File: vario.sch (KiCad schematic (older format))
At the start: 177 parts, among them J10 Conn_01x06, J11 Conn_01x04, J12 Conn_01x04, J13 Conn_01x04, J14 Conn_01x03, J15 Conn_01x04, J16 Conn_01x06, J17 Conn_01x06, J18 Conn_01x04, J19 Conn_01x04, J2 Conn_01x02, J20 Conn_01x06, J21 Conn_Coaxial, J22 USB_B_Micro, J23 USB_B_Micro, J24 Micro_SD_Card_Det_Hirose_DM3AT, J3 6339167-3, J6 Conn_01x06, J7 Conn_01x04, J8 Conn_01x04, J9 Conn_01x02, Q1 AO3401A, SW1 SW_MEC_5E, U1 STM32F407VGTx, U10 AMS1117-3.3, U11 HSCMRRN001PD2A3, U12 MS5611-01BA, U13 MAX3232ECPWR, U14 BLE_HM-11, U15 USBLC6-2SC6, U16 USBLC6-2SC6, U17 AMS1117-3.3, U18 HAMMOND_1593W, U2 MP2359DJ-LF-Z, U3 MP2359DJ-LF-Z, U4 L3GD20, U5 MTi-1IMU, U6 FXOS8700, U7 MS5611-01BA, U8 NEO-M9N, U9 TCAN332DR, Y1 16MHz

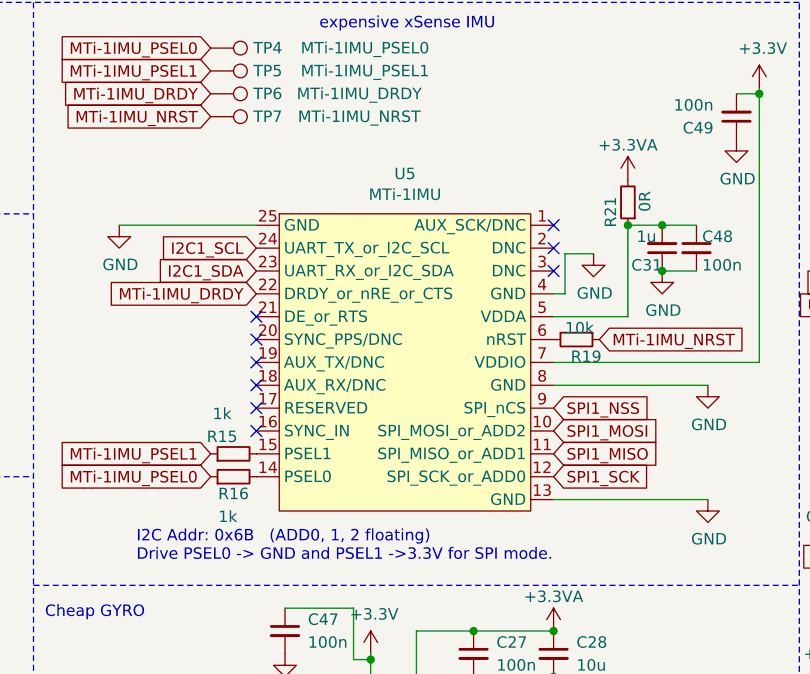
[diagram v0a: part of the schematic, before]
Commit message: added latest Schematic file.
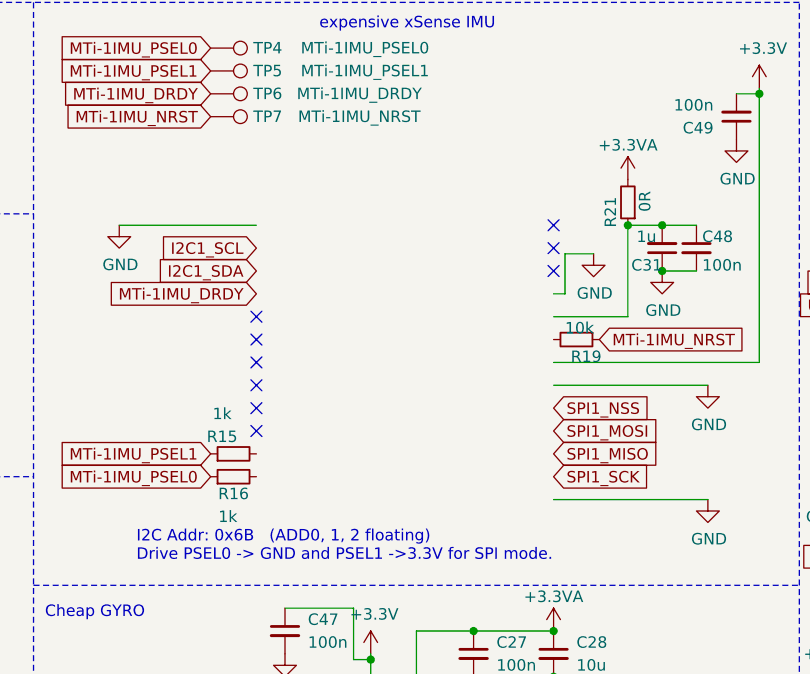
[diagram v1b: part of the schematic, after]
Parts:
- removed U5: MTi-1IMU, OWN_Parts_:XSens_MTi1_IMU, symbol OWN_Parts_:MTi-1IMU
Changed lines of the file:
@@
-$EndComp
-$Comp
-L OWN_Parts_:MTi-1IMU U5
-U 1 1 5F93C09B
-P 8025 3675
-F 0 "U5" H 8025 4450 50  0000 C CNN
-F 1 "MTi-1IMU" H 8025 4359 50  0000 C CNN
-F 2 "OWN_Parts_:XSens_MTi1_IMU" H 8125 4475 50  0001 C CNN
-F 3 "" H 8125 4475 50  0001 C CNN
-F 4 "512-MTI-1T" H 8025 3675 50  0001 C CNN "Mouser Part Number"
-F 5 "512-MTI-1T" H 8025 3675 50  0001 C CNN "Mouser-Nr.:"
-	1    8025 3675
-	1    0    0    -1
 $EndComp
 $Comp
